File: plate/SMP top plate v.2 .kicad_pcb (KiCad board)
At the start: 2 copper layers, 114.7 x 58.7 mm, 4 parts

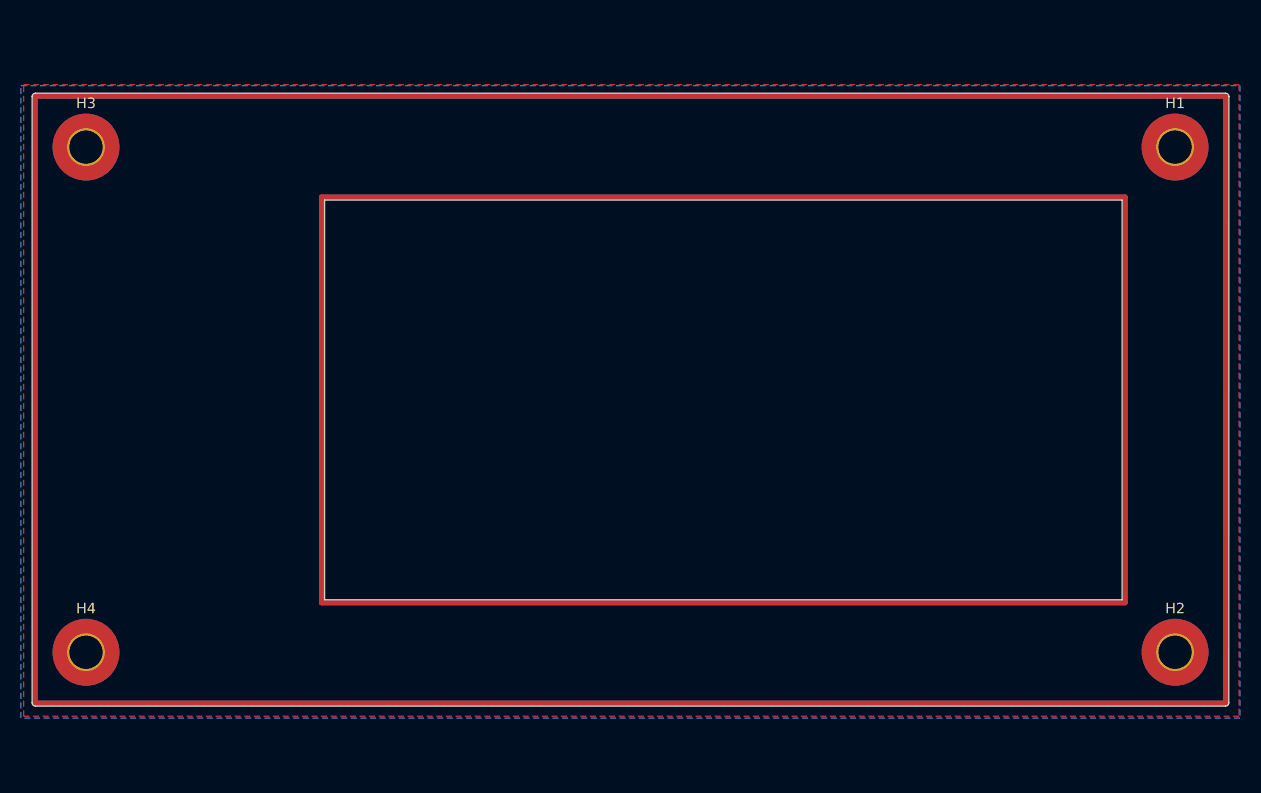
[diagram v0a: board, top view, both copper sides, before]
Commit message: pcb and plate finalize for v.4
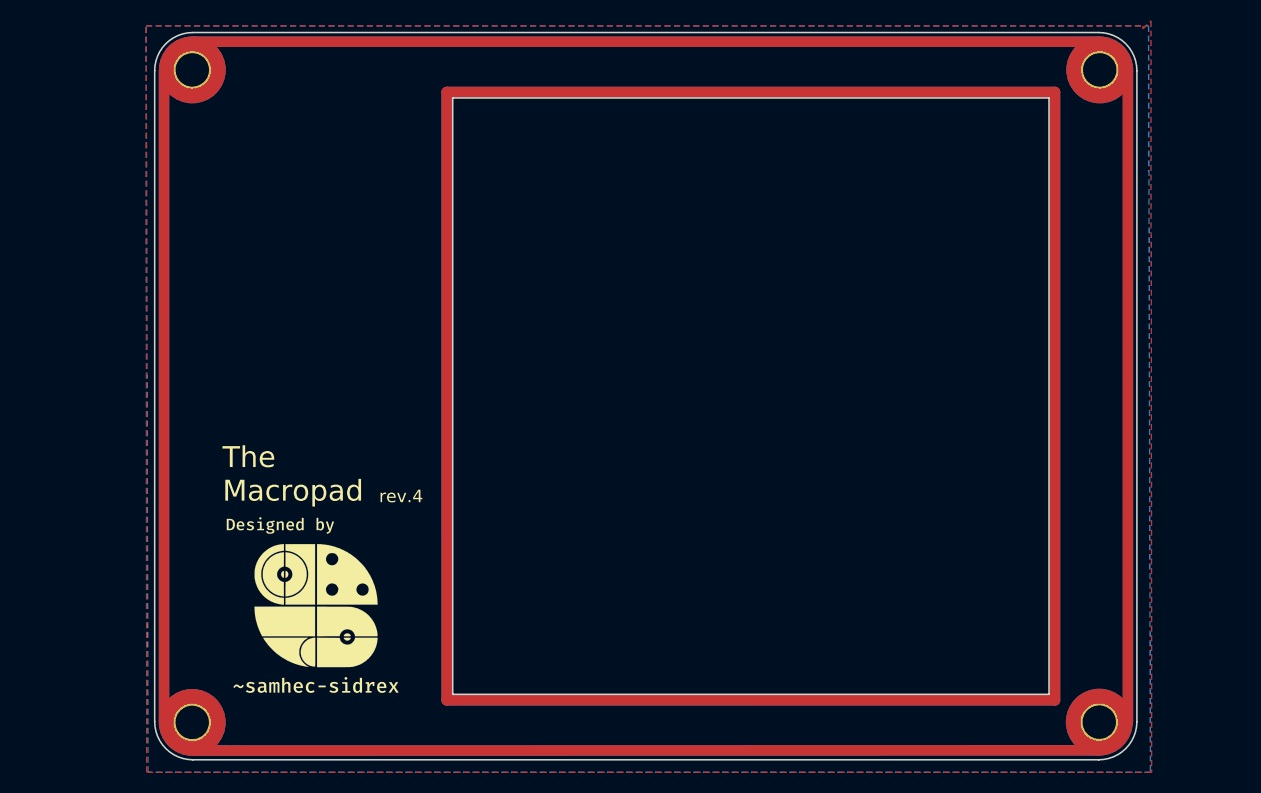
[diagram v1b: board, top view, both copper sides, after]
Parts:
- added Ref**: Val**, 8hands:urbit-sigil-silks, F.Cu at (106.7, 120.3)
- added kibuzzard-6147B285: G***, label, F.Cu at (106.7, 127.9)
- added kibuzzard-6147B2C4: G***, label, F.Cu at (103.3, 112.6)
- moved H4 97.3 mm to (181.8, 131.5)
- moved H1 94.5 mm to (94.9, 69.0)
- moved H2 56.3 mm to (181.8, 69.0)
- moved H3 56.1 mm to (94.9, 131.5)
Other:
- board size 114.7 x 58.7 mm -> 94.1 x 69.7 mm
- board text added: "The Macropad"
- board text added: "rev.4"
